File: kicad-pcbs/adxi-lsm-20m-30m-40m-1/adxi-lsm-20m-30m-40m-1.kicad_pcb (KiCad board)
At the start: 2 copper layers, 128.4 x 71.1 mm, 54 parts, among them J1 ANT, J2 Conn_01x04, J3 Conn_01x04, J4 Conn_01x04

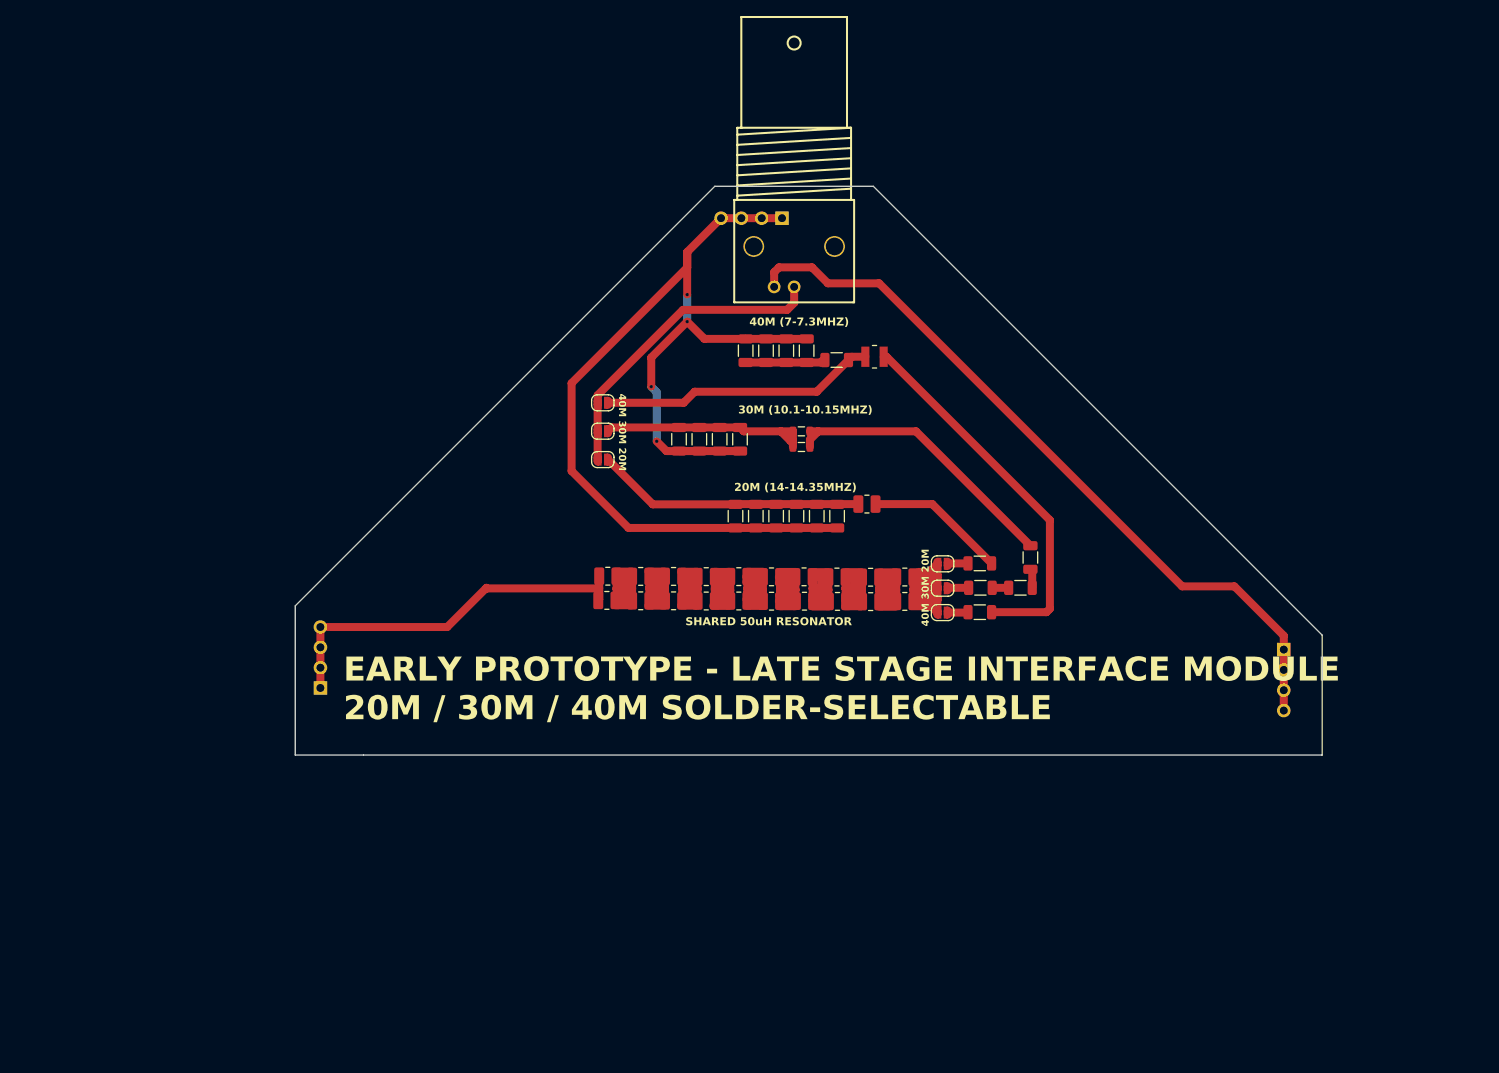
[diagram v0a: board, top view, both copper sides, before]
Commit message: 20m/30m/40m late stage module
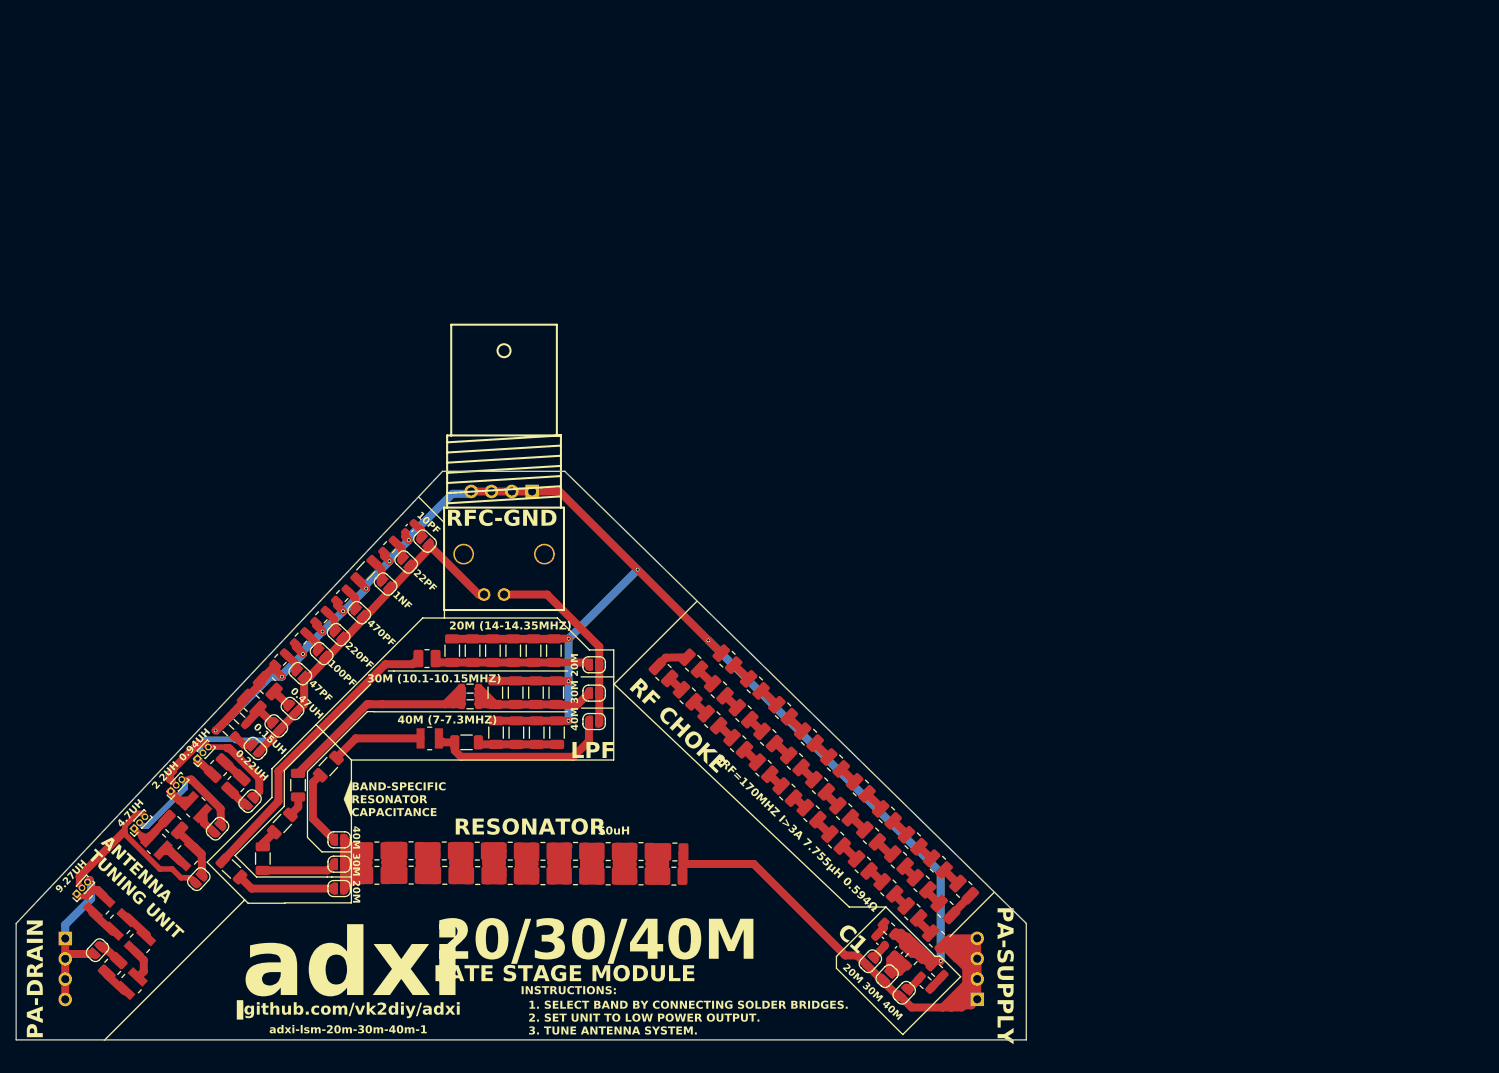
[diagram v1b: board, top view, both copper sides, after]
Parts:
- added C1: 10pF, Capacitor_SMD:C_0603_1608Metric, F.Cu at (103.0, 71.1)
- added C10: 100pF, Capacitor_SMD:C_0805_2012Metric, F.Cu at (89.5, 84.9)
- added C15: 220pF, Capacitor_SMD:C_0805_2012Metric, F.Cu at (92.0, 82.2)
- added C26: 470pF, Capacitor_SMD:C_0805_2012Metric, F.Cu at (94.6, 79.6)
- added C27: 1nF, Capacitor_SMD:C_1206_3216Metric, F.Cu at (97.6, 76.4)
- added C28: 100pF, Capacitor_SMD:C_0805_2012Metric, F.Cu at (163.0, 121.2)
- added C29: 12pF, Capacitor_SMD:C_0603_1608Metric, F.Cu at (164.2, 123.9)
- added C30: 68pF, Capacitor_SMD:C_0603_1608Metric, F.Cu at (161.9, 122.7)
- added C31: 100pF, Capacitor_SMD:C_0805_2012Metric, F.Cu at (167.5, 127.9)
- added C32: 470pF, Capacitor_SMD:C_0805_2012Metric, F.Cu at (169.0, 126.4)
- added C33: 47pF, Capacitor_SMD:C_0805_2012Metric, F.Cu at (165.8, 125.0)
- added C5: 22pF, Capacitor_SMD:C_0805_2012Metric, F.Cu at (100.5, 73.5)
- added C9: 47pF, Capacitor_SMD:C_0805_2012Metric, F.Cu at (86.9, 87.6)
- added JP10: 100PF, Jumper:SolderJumper-2_P1.3mm_Open_RoundedPad1.0x1.5mm, F.Cu at (92.0, 86.8)
- added JP11: 220PF, Jumper:SolderJumper-2_P1.3mm_Open_RoundedPad1.0x1.5mm, F.Cu at (94.2, 84.4)
- added JP12: 470PF, Jumper:SolderJumper-2_P1.3mm_Open_RoundedPad1.0x1.5mm, F.Cu at (96.8, 81.7)
- added JP13: 1NF, Jumper:SolderJumper-2_P1.3mm_Open_RoundedPad1.0x1.5mm, F.Cu at (100.0, 78.1)
- added JP14: 0.15UH, Jumper:SolderJumper-2_P1.3mm_Open_RoundedPad1.0x1.5mm, F.Cu at (86.4, 95.8)
- added JP15: 0.22UH, Jumper:SolderJumper-2_P1.3mm_Open_RoundedPad1.0x1.5mm, F.Cu at (83.8, 98.6)
- added JP16: 0.47UH, Jumper:SolderJumper-2_P1.3mm_Open_RoundedPad1.0x1.5mm, F.Cu at (88.4, 93.7)
- added JP17: 0.94UH, Connector_PinHeader_1.00mm:PinHeader_1x03_P1.00mm_Vertical, F.Cu at (76.5, 99.9)
- added JP18: 2.2UH, Connector_PinHeader_1.00mm:PinHeader_1x03_P1.00mm_Vertical, F.Cu at (73.2, 104.0)
- added JP19: 9.27UH, Connector_PinHeader_1.00mm:PinHeader_1x03_P1.00mm_Vertical, F.Cu at (61.4, 116.8)
- added JP20: 40M, Jumper:SolderJumper-2_P1.3mm_Open_RoundedPad1.0x1.5mm, F.Cu at (164.9, 129.2)
- added JP21: 0.94UH., Jumper:SolderJumper-2_P1.3mm_Open_RoundedPad1.0x1.5mm, F.Cu at (83.1, 105.2)
- added JP22: 2.2UH., Jumper:SolderJumper-2_P1.3mm_Open_RoundedPad1.0x1.5mm, F.Cu at (79.0, 108.7)
- added JP23: 4.7UH., Jumper:SolderJumper-2_P1.3mm_Open_RoundedPad1.0x1.5mm, F.Cu at (76.7, 115.0)
- added JP24: 9.27UH., Jumper:SolderJumper-2_P1.3mm_Open_RoundedPad1.0x1.5mm, F.Cu at (64.0, 123.9)
- added JP25: 4.7UH, Connector_PinHeader_1.00mm:PinHeader_1x03_P1.00mm_Vertical, F.Cu at (68.6, 108.6)
- added JP26: 30M, Jumper:SolderJumper-2_P1.3mm_Open_RoundedPad1.0x1.5mm, F.Cu at (162.7, 127.1)
- added JP27: 20M, Jumper:SolderJumper-2_P1.3mm_Open_RoundedPad1.0x1.5mm, F.Cu at (160.6, 125.2)
- added JP7: 10PF, Jumper:SolderJumper-2_P1.3mm_Open_RoundedPad1.0x1.5mm, F.Cu at (105.0, 72.7)
- added JP8: 22PF, Jumper:SolderJumper-2_P1.3mm_Open_RoundedPad1.0x1.5mm, F.Cu at (102.6, 75.3)
- added JP9: 47PF, Jumper:SolderJumper-2_P1.3mm_Open_RoundedPad1.0x1.5mm, F.Cu at (89.4, 89.3)
- added L25: 470nH, Inductor_SMD:L_1008_2520Metric, F.Cu at (169.0, 122.5)
- added L26: 470nH, Inductor_SMD:L_1008_2520Metric, F.Cu at (165.9, 119.1)
- added L27: 470nH, Inductor_SMD:L_1008_2520Metric, F.Cu at (162.9, 116.1)
- added L28: 470nH, Inductor_SMD:L_1008_2520Metric, F.Cu at (159.7, 113.2)
- added L29: 470nH, Inductor_SMD:L_1008_2520Metric, F.Cu at (156.4, 110.1)
- added L30: 470nH, Inductor_SMD:L_1008_2520Metric, F.Cu at (153.3, 106.8)
- added L31: 470nH, Inductor_SMD:L_1008_2520Metric, F.Cu at (150.3, 104.1)
- added L32: 470nH, Inductor_SMD:L_1008_2520Metric, F.Cu at (147.3, 101.1)
- added L33: 470nH, Inductor_SMD:L_1008_2520Metric, F.Cu at (144.1, 98.1)
- added L34: 470nH, Inductor_SMD:L_1008_2520Metric, F.Cu at (140.9, 95.0)
- added L35: 470nH, Inductor_SMD:L_1008_2520Metric, F.Cu at (137.8, 92.1)
- added L36: 470nH, Inductor_SMD:L_1008_2520Metric, F.Cu at (134.8, 89.1)
- added L37: 470nH, Inductor_SMD:L_1008_2520Metric, F.Cu at (138.5, 88.0)
- added L38: 470nH, Inductor_SMD:L_1008_2520Metric, F.Cu at (141.7, 91.3)
- added L39: 470nH, Inductor_SMD:L_1008_2520Metric, F.Cu at (144.8, 94.3)
- added L40: 470nH, Inductor_SMD:L_1008_2520Metric, F.Cu at (147.9, 97.3)
- added L41: 470nH, Inductor_SMD:L_1008_2520Metric, F.Cu at (151.2, 100.3)
- added L42: 470nH, Inductor_SMD:L_1008_2520Metric, F.Cu at (154.4, 103.3)
- added L43: 470nH, Inductor_SMD:L_1008_2520Metric, F.Cu at (157.4, 106.5)
- added L44: 470nH, Inductor_SMD:L_1008_2520Metric, F.Cu at (160.7, 109.6)
- added L45: 470nH, Inductor_SMD:L_1008_2520Metric, F.Cu at (164.2, 112.6)
- added L46: 470nH, Inductor_SMD:L_1008_2520Metric, F.Cu at (167.0, 115.6)
- added L47: 470nH, Inductor_SMD:L_1008_2520Metric, F.Cu at (170.0, 118.8)
- added L48: 470nH, Inductor_SMD:L_1008_2520Metric, F.Cu at (172.4, 116.3)
- added L49: 470nH, Inductor_SMD:L_1008_2520Metric, F.Cu at (169.1, 113.1)
- added L50: 470nH, Inductor_SMD:L_1008_2520Metric, F.Cu at (165.9, 110.2)
- added L51: 470nH, Inductor_SMD:L_1008_2520Metric, F.Cu at (162.7, 107.0)
- added L52: 470nH, Inductor_SMD:L_1008_2520Metric, F.Cu at (159.4, 103.6)
- added L53: 470nH, Inductor_SMD:L_1008_2520Metric, F.Cu at (156.2, 100.5)
- added L54: 470nH, Inductor_SMD:L_1008_2520Metric, F.Cu at (153.0, 97.2)
- added L55: 470nH, Inductor_SMD:L_1008_2520Metric, F.Cu at (149.7, 93.9)
- added L56: 470nH, Inductor_SMD:L_1008_2520Metric, F.Cu at (146.2, 90.7)
- added L57: 470nH, Inductor_SMD:L_1008_2520Metric, F.Cu at (142.8, 87.5)
- added L58: 470nH, Inductor_SMD:L_1008_2520Metric, F.Cu at (83.3, 93.0)
- added L59: 220nH, Inductor_SMD:L_0805_2012Metric, F.Cu at (81.8, 94.9)
- added L60: 220nH, Inductor_SMD:L_0805_2012Metric, F.Cu at (80.4, 96.4)
- added L61: 470nH, Inductor_SMD:L_1008_2520Metric, F.Cu at (85.3, 90.8)
- added L62: 470nH, Inductor_SMD:L_1008_2520Metric, F.Cu at (79.2, 101.1)
- added L63: 470nH, Inductor_SMD:L_1008_2520Metric, F.Cu at (81.3, 103.1)
- added L64: 2.2uH, adxi-footprints:L_Chilisin_NLC252018-2.92x2.50x2.20, F.Cu at (76.4, 106.0)
- added L65: 2.2uH, adxi-footprints:L_Chilisin_NLC252018-2.92x2.50x2.20, F.Cu at (71.4, 110.6)
- added L66: 2.2uH, adxi-footprints:L_Chilisin_NLC252018-2.92x2.50x2.20, F.Cu at (75.3, 111.9)
- added L67: 470nH, Inductor_SMD:L_1008_2520Metric, F.Cu at (73.5, 108.1)
- added L68: 2.2uH, adxi-footprints:L_Chilisin_NLC252018-2.92x2.50x2.20, F.Cu at (64.2, 118.2)
- added L69: 2.2uH, adxi-footprints:L_Chilisin_NLC252018-2.92x2.50x2.20, F.Cu at (66.9, 120.6)
- added L70: 2.2uH, adxi-footprints:L_Chilisin_NLC252018-2.92x2.50x2.20, F.Cu at (69.3, 123.0)
- added L71: 2.2uH, adxi-footprints:L_Chilisin_NLC252018-2.92x2.50x2.20, F.Cu at (68.3, 128.1)
- added L72: 470nH, Inductor_SMD:L_1008_2520Metric, F.Cu at (65.9, 125.9)
- J2: value Conn_01x04 -> PA-DRAIN
- J3: value Conn_01x04 -> PA-SUPPLY
- J4: value Conn_01x04 -> RFC-GND
- moved J2 156.5 mm to (60.0, 122.4)
- moved C7 101.0 mm to (80.8, 113.7), turned to 137 degrees
- moved C12 96.9 mm to (87.1, 108.0), turned to 47 degrees
- moved C11 95.9 mm to (84.7, 112.4), turned to 90 degrees
- moved C13 95.9 mm to (89.1, 103.2)
- moved J3 90.9 mm to (174.0, 130.0)
- moved JP1 85.7 mm to (94.2, 116.2), turned to 180 degrees
- moved C14 83.7 mm to (92.9, 100.9), turned to 47 degrees
- moved JP2 82.9 mm to (94.2, 113.1), turned to 180 degrees
- moved JP3 80.6 mm to (94.2, 110.1), turned to 180 degrees
- moved L21 75.8 mm to (99.0, 114.5), turned to 180 degrees
- moved L11 73.2 mm to (105.6, 97.4), turned to 0 degrees
- moved L16 73.0 mm to (99.0, 111.5), turned to 180 degrees
- moved L20 68.4 mm to (103.2, 114.5), turned to 180 degrees
- moved C3 66.5 mm to (110.2, 97.9), turned to 0 degrees
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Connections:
- J2 pad 1: Net-(J1-Ext) -> Net-(J2-Pin_1)
- J2 pad 2: Net-(J1-Ext) -> Net-(J2-Pin_1)
- J2 pad 3: Net-(J1-Ext) -> Net-(J2-Pin_1)
- J2 pad 4: Net-(J1-Ext) -> Net-(J2-Pin_1)
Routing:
- net /GND: track 143.3 -> 233.8 mm, vias 4 -> 14
- net Net-(J3-Pin_1): track 47.6 -> 114.4 mm
- net Net-(J1-Ext): track 94.2 -> 54.4 mm, vias 0 -> 1
- net Net-(C14-Pad2): track 47.8 -> 11.6 mm
- net Net-(JP19-Pin_2): track 0.00 -> 25.1 mm
- net Net-(J2-Pin_1): track 0.00 -> 20.4 mm
- net Net-(C7-Pad2): track 17.6 -> 37.3 mm
- net Net-(JP17-Pin_3): track 0.00 -> 19.0 mm
- net Net-(JP18-Pin_3): track 0.00 -> 17.5 mm
- net Net-(J1-In): track 39.4 -> 24.0 mm
- net Net-(JP4-A): track 33.6 -> 19.5 mm
- net Net-(JP6-A): track 34.5 -> 23.6 mm
- net Net-(JP1-B): track 2.55 -> 12.3 mm
- net Net-(JP26-A): track 0.00 -> 9.59 mm
- net Net-(JP3-B): track 2.55 -> 9.61 mm
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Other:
- board size 128.4 x 71.1 mm -> 126.3 x 71.1 mm
- board text added: "("
- board text added: "0.15UH"
- board text added: "0.22UH"
- board text added: "0.47UH"
- board text added: "0.94UH"
- board text added: "1. SELECT BAND BY CONNECTING SOLDER BRIDGES. 2. SET UNIT TO LOW POWER OUTPUT. 3. TUNE ANTENNA SYSTEM."
- board text added: "100PF"
- board text added: "10PF"
- board text added: "1NF"
- board text added: "2.2UH"
- board text added: "20/30/40M"
- board text added: "20M 30M 40M"
- board text added: "220PF"
- board text added: "22PF"
- board text added: "4.7UH"
- board text added: "470PF"
- board text added: "47PF"
- board text added: "50uH"
- board text added: "9.27UH"
- board text added: "ANTENNA TUNING UNIT"
- board text added: "BAND-SPECIFIC RESONATOR CAPACITANCE"
- board text added: "C1"
- board text added: "INSTRUCTIONS:"
- board text added: "KEEP CLEAR OF METAL"
- board text added: "LATE STAGE MODULE"
- board text added: "LPF"
- board text added: "PA-DRAIN"
- board text added: "PA-SUPPLY"
- board text added: "RESONANCE ZONE"
- board text added: "RESONATOR"
- board text added: "RF CHOKE"
- board text added: "RFC-GND"
- board text added: "SRF=170MHZ I>3A 7.755μH 0.594Ω"
- board text added: "adxi"
- board text added: "adxi-lsm-20m-30m-40m-1"
- board text added: "github.com/vk2diy/adxi"
- board text removed: "EARLY PROTOTYPE - LATE STAGE INTERFACE MODULE 20M / 30M / 40M SOLDER-SELECTABLE"
- board text removed: "SHARED 50uH RESONATOR"
